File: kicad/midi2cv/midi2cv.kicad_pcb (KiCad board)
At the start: 2 copper layers, 81.3 x 96.5 mm, 61 parts, among them J1 ProgramJmpr, J10 CTL1 Output, J11 CTL2 Output, J12 Gate1 Output, J13 Gate2 Output, J14 Conn_01x08_Male, J15 Conn_01x08_Female, J16 P1, J17 P2, J18 P3, J19 P4, J2 Power, J20 P5, J21 P6, J22 P7, J23 P8, J3 Conn_01x04_Male, J4 Conn_01x04_Female, J5 Conn_01x08_Male, J6 Conn_01x08_Female, J7 Midi Input, J8 CV1 Output, J9 CV2 Output, U1 L7805, U2 24LC256, U3 MCP4922, U4 MCP4922, U5 PC817, U6 TL074, U7 74HC595, U8 TL074

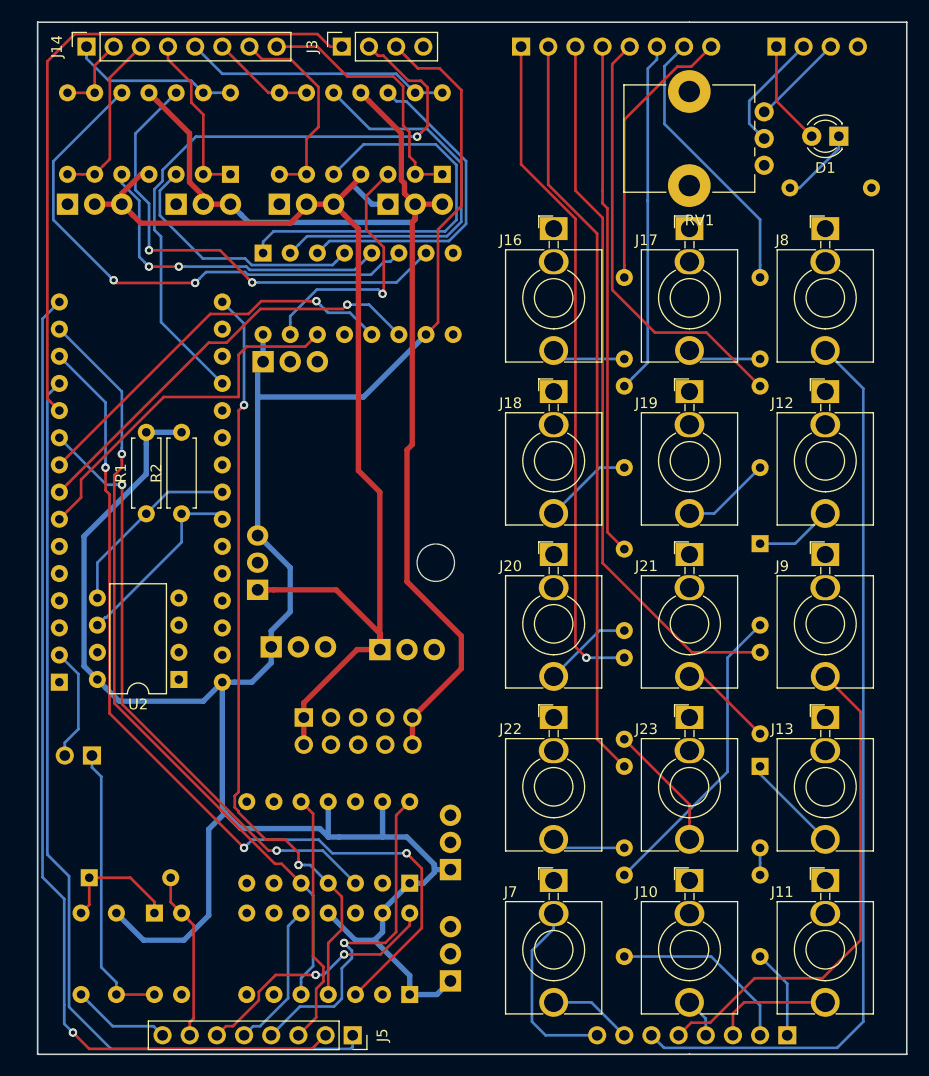
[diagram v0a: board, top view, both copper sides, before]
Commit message: Create pcb.
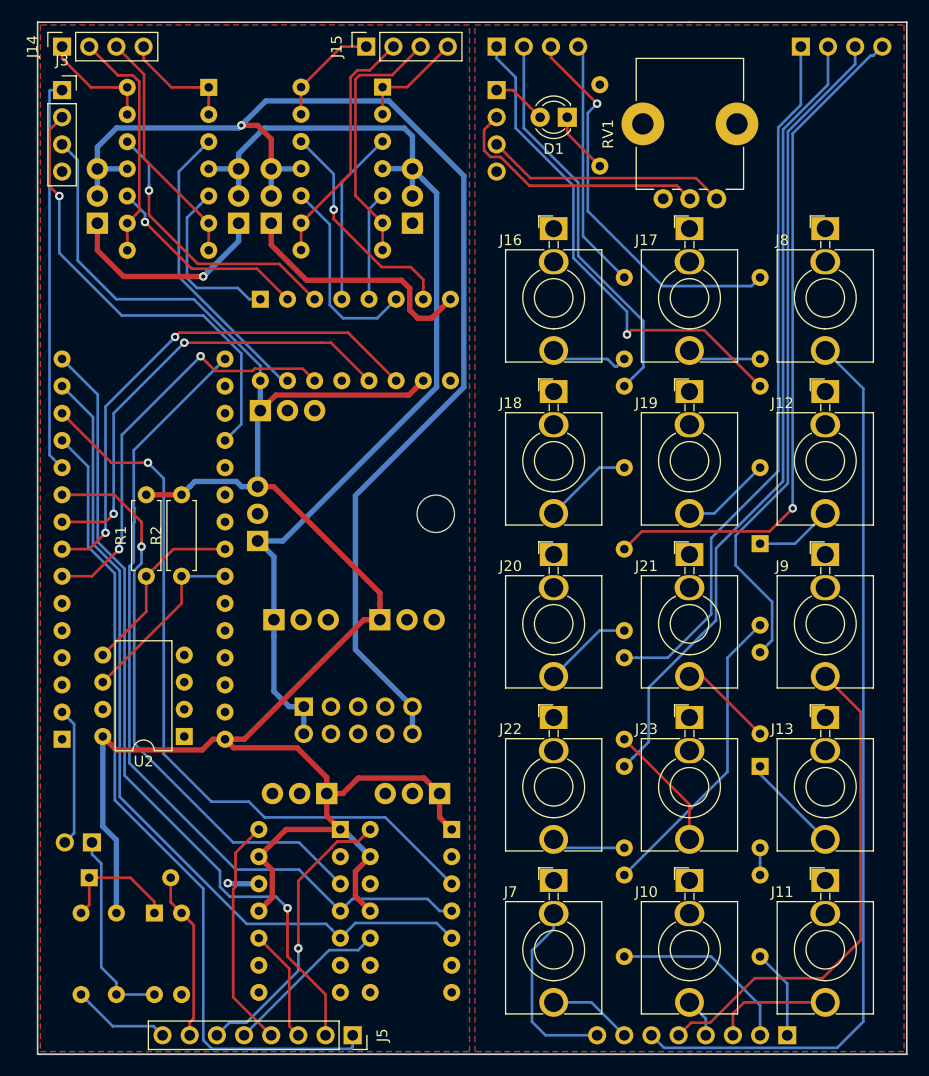
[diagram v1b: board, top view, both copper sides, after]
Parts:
- added J24: Conn_01x04_Female, Connector_PinHeader_2.54mm:PinHeader_1x04_P2.54mm_Vertical, B.Cu at (73.4, 32.8)
- added J25: Conn_01x04_Female, Connector_PinHeader_2.54mm:PinHeader_1x04_P2.54mm_Vertical, B.Cu at (101.9, 32.8)
- J14: value Conn_01x08_Male -> Conn_01x04_Male; footprint Connector_PinSocket_2.54mm:PinSocket_1x08_P2.54mm_Vertical -> Connector_PinSocket_2.54mm:PinSocket_1x04_P2.54mm_Vertical
- J15: value Conn_01x08_Female -> Conn_01x04_Male; footprint Connector_PinHeader_2.54mm:PinHeader_1x08_P2.54mm_Vertical -> Connector_PinSocket_2.54mm:PinSocket_1x04_P2.54mm_Vertical; moved to F.Cu
- moved C8 30.8 mm to (66.5, 46.7), turned to 90 degrees
- moved C6 28.8 mm to (37.1, 46.7), turned to 90 degrees
- moved J3 26.5 mm to (32.8, 36.8), turned to 0 degrees
- moved J4 26.5 mm to (73.4, 36.8), turned to 180 degrees
- moved D1 25.5 mm to (80.0, 39.4)
- moved U6 23.3 mm to (46.5, 36.6), turned to 180 degrees
- moved R3 17.9 mm to (83.1, 43.9), turned to 90 degrees
- moved C4 16.6 mm to (65.5, 101.6), turned to 180 degrees
- moved U8 16.4 mm to (62.7, 36.6), turned to 180 degrees
- moved C3 16.1 mm to (55.0, 101.6), turned to 180 degrees
- moved U3 15.9 mm to (69.2, 106.0), turned to 180 degrees
- moved J15 14.5 mm to (61.2, 32.8), turned to 90 degrees
- moved C2 10.5 mm to (65.0, 87.4)
- moved C1 10.3 mm to (55.1, 87.4)
- moved RV1 9.26 mm to (94.0, 47.0), turned to 90 degrees
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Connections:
- R10 pad 1: Net-(J15-Pad6) -> Net-(J24-Pad2)
- R11 pad 1: Net-(J15-Pad5) -> Net-(J24-Pad1)
- R12 pad 1: Net-(J15-Pad4) -> Net-(J25-Pad4)
- R13 pad 1: Net-(J15-Pad3) -> Net-(J25-Pad3)
- R14 pad 1: Net-(J15-Pad2) -> Net-(J25-Pad2)
- R15 pad 1: Net-(J15-Pad1) -> Net-(J25-Pad1)
- R8 pad 1: Net-(J15-Pad8) -> Net-(J24-Pad4)
- R9 pad 1: Net-(J15-Pad7) -> Net-(J24-Pad3)
- U6 pad 1: Net-(J14-Pad8) -> Net-(J14-Pad4)
- U6 pad 13: Net-(J14-Pad5) -> Net-(J14-Pad1)
- U6 pad 14: Net-(J14-Pad5) -> Net-(J14-Pad1)
- U6 pad 2: Net-(J14-Pad8) -> Net-(J14-Pad4)
- U6 pad 6: Net-(J14-Pad7) -> Net-(J14-Pad3)
- U6 pad 7: Net-(J14-Pad7) -> Net-(J14-Pad3)
- U6 pad 8: Net-(J14-Pad6) -> Net-(J14-Pad2)
- U6 pad 9: Net-(J14-Pad6) -> Net-(J14-Pad2)
- U8 pad 1: Net-(J14-Pad4) -> Net-(J15-Pad4)
- U8 pad 13: Net-(J14-Pad1) -> Net-(J15-Pad1)
- U8 pad 14: Net-(J14-Pad1) -> Net-(J15-Pad1)
- U8 pad 2: Net-(J14-Pad4) -> Net-(J15-Pad4)
- U8 pad 6: Net-(J14-Pad3) -> Net-(J15-Pad3)
- U8 pad 7: Net-(J14-Pad3) -> Net-(J15-Pad3)
- U8 pad 8: Net-(J14-Pad2) -> Net-(J15-Pad2)
- U8 pad 9: Net-(J14-Pad2) -> Net-(J15-Pad2)
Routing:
- net Net-(J25-Pad2): track 0.00 -> 75.2 mm
- net Net-(J25-Pad1): track 0.00 -> 66.4 mm
- net Net-(J25-Pad4): track 0.00 -> 64.1 mm, vias 0 -> 1
- net Net-(J25-Pad3): track 0.00 -> 63.2 mm
- net Net-(J15-Pad1): track 63.2 -> 10.2 mm, vias 1 -> 0
- net Net-(J15-Pad2): track 70.3 -> 23.3 mm
- net Net-(J24-Pad1): track 0.00 -> 46.8 mm, vias 0 -> 1
- net GND: track 3.66 -> 47.0 mm, vias 0 -> 2
- net Net-(J15-Pad3): track 67.5 -> 24.4 mm
- net Net-(J15-Pad5): track 41.0 -> 0.00 mm
- net Net-(J15-Pad4): track 47.8 -> 10.2 mm
- net Net-(J24-Pad2): track 0.00 -> 37.1 mm
- net Net-(J24-Pad3): track 0.00 -> 36.9 mm, vias 0 -> 1
- net Net-(J15-Pad6): track 33.2 -> 0.00 mm
- net Net-(U7-Pad6): track 50.7 -> 18.8 mm, vias 2 -> 0
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- added copper zone on F.Cu, net GND
- added copper zone on F.Cu, net GNDA
